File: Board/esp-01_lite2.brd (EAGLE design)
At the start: 17.4 x 56.8 mm, 26 parts, among them IC1 TINY13-20SU, K1 setup, K2 reset, X1 235-102, X2 235-102

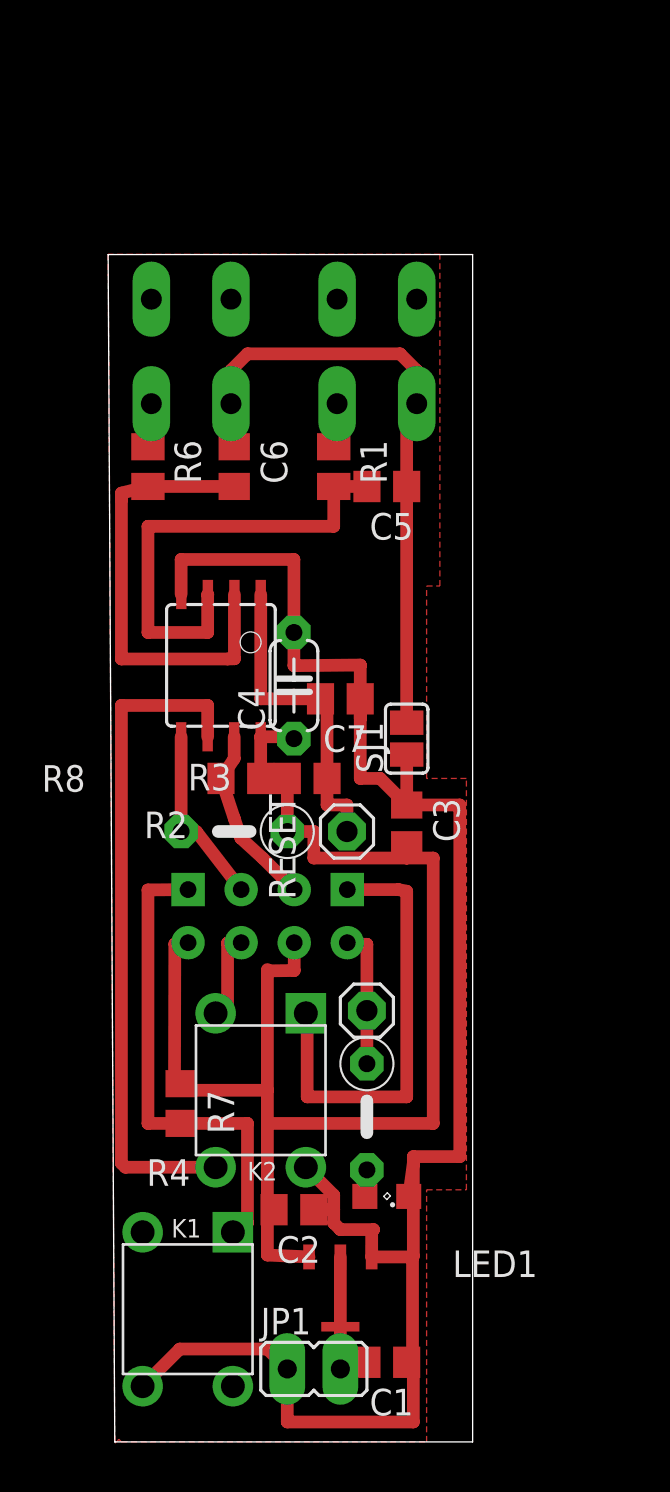
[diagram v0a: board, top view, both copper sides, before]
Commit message: LED works, server ok, ESP 24h
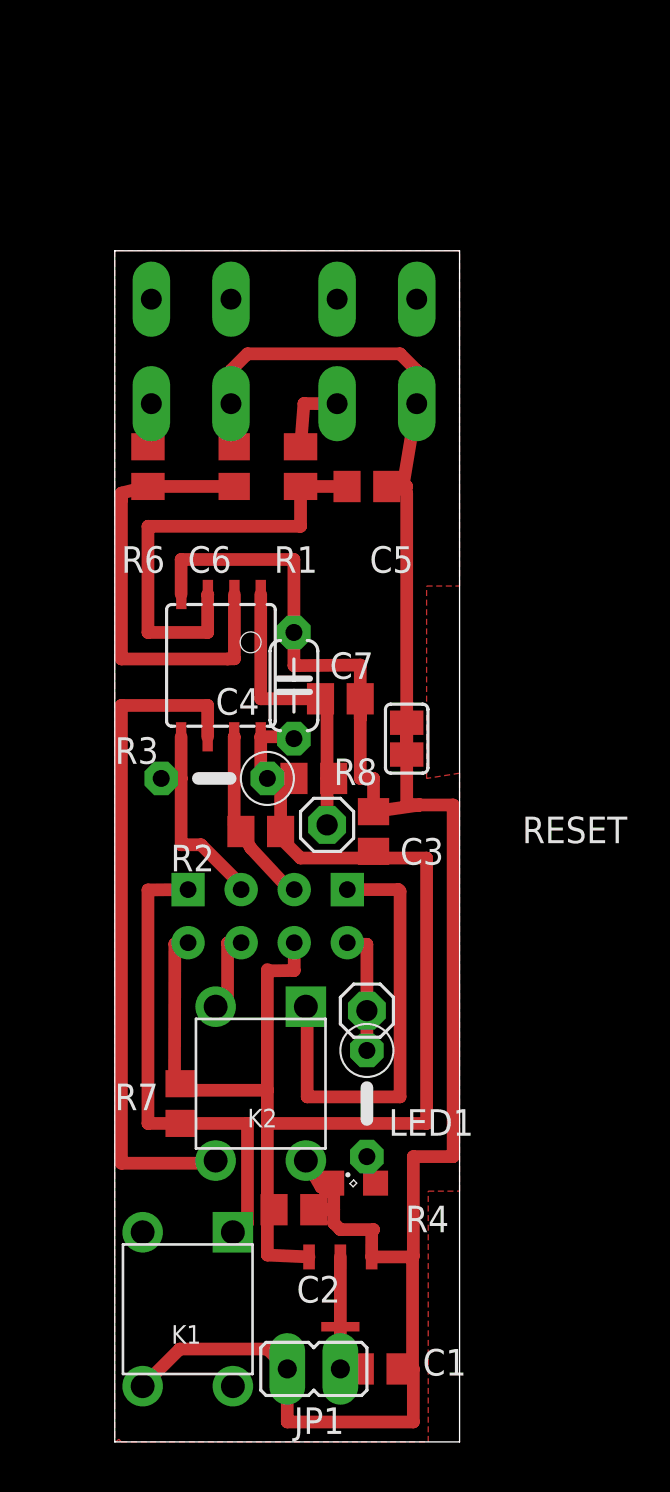
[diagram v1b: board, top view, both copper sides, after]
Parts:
- moved R2 2.71 mm to (6.99, 29.2)
- moved R3 2.71 mm to (4.76, 31.8)
- moved LED1 1.71 mm to (11.4, 12.4), turned to 0 degrees
- moved C3 1.62 mm to (12.4, 29.2)
- moved R1 1.59 mm to (8.89, 46.7)
- moved RESET 1.00 mm to (10.2, 29.5), turned to 90 degrees
- moved C5 0.95 mm to (12.1, 45.7)
- moved R4 0.63 mm to (12.1, 16.2)
- moved C1 0.45 mm to (12.7, 3.49)
- moved R8 0.32 mm to (9.53, 31.8)
- moved K2 0.32 mm to (6.99, 17.1)
- turned SJ1 to 270 degrees
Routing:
- net N$5: track 30.3 -> 34.4 mm
- net GND: track 90.3 -> 93.4 mm
- net N$4: track 2.09 -> 3.66 mm
- net SDA: track 8.77 -> 10.0 mm
- net IN2: track 22.1 -> 21.2 mm
- net N$13: track 16.2 -> 15.2 mm
- net LOG: track 6.66 -> 6.03 mm
- net +3V3: track 68.0 -> 67.4 mm
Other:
- board size 17.4 x 56.8 mm -> 16.5 x 57 mm

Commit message: new board
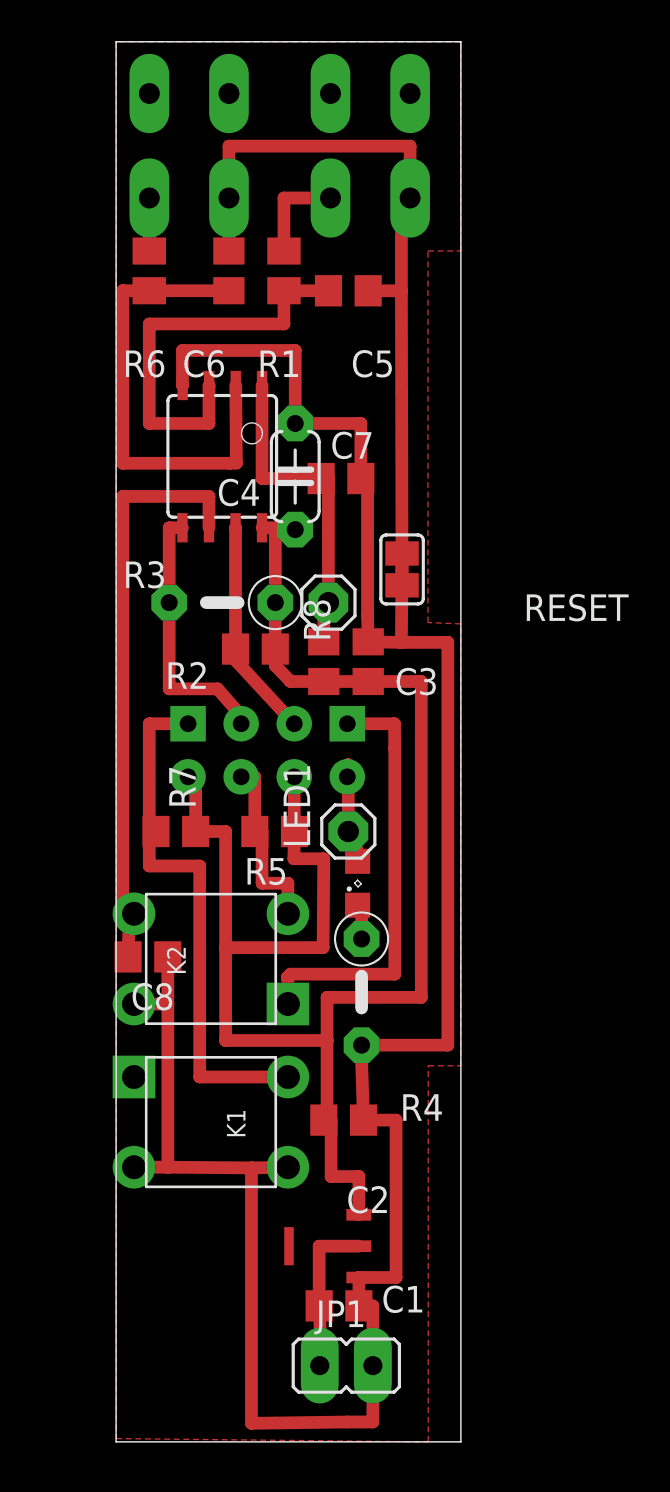
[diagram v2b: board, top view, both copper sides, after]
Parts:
- added C8: 0.1, resistor:C0805
- added R5: 10k, rcl:R0805
- moved LED1 14.4 mm to (11.6, 26.7), turned to 90 degrees
- moved R7 13.0 mm to (2.92, 29.2), turned to 180 degrees
- moved RESET 10.6 mm to (10.2, 40.2)
- moved C7 10.5 mm to (10.8, 46.1)
- moved C4 10.0 mm to (8.64, 46.2)
- moved IC1 10.0 mm to (5.14, 47.1)
- moved X2 9.85 mm to (12.4, 62.9)
- moved X1 9.84 mm to (3.71, 62.9)
- moved C5 9.41 mm to (11.2, 55.1)
- moved R1 9.40 mm to (8.10, 56.0)
- moved C6 9.37 mm to (5.46, 56.0)
- moved R6 9.37 mm to (1.65, 56.0)
- moved K1 9.02 mm to (4.60, 15.3), turned to 0 degrees
- moved R2 8.73 mm to (6.73, 37.9)
- moved LOG 8.62 mm to (11.2, 29.2)
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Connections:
- removed net LOG: LOG.1, R4.1, U$1.TX
- removed net N$12: LED1.A, R4.2
- new net N$1: LED1.A, LOG.1, U$1.TX
- new net N$6: LED1.C, R4.1
- net +3V3: now also R5.1
- net GND: now also C8.1, K1.2, R4.2; no longer LED1.C
- net N$2: now also R5.2
- net RX: now also K1.4; no longer K1.1
- net WAKE_UP: now also C8.2
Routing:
- net GND: track 93.4 -> 114.9 mm
- net +3V3: track 67.4 -> 81.7 mm
- net LOG: track 6.03 -> 0.00 mm
- net N$1: track 0.00 -> 5.31 mm
- net N$2: track 4.34 -> 8.79 mm
- net WAKE_UP: track 32.1 -> 28.4 mm
- net SDA: track 10.0 -> 12.7 mm
- net N$5: track 34.4 -> 36.7 mm
- net RX: track 23.5 -> 25.7 mm
- net SCK: track 8.72 -> 10.5 mm
- net N$6: track 0.00 -> 1.69 mm
- net IN2: track 21.2 -> 19.6 mm
- net AA*3: track 6.31 -> 7.71 mm
- net N$12: track 1.35 -> 0.00 mm
- net N$4: track 3.66 -> 4.76 mm
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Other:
- board size 16.5 x 57 mm -> 16.5 x 67 mm

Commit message: board for one_button
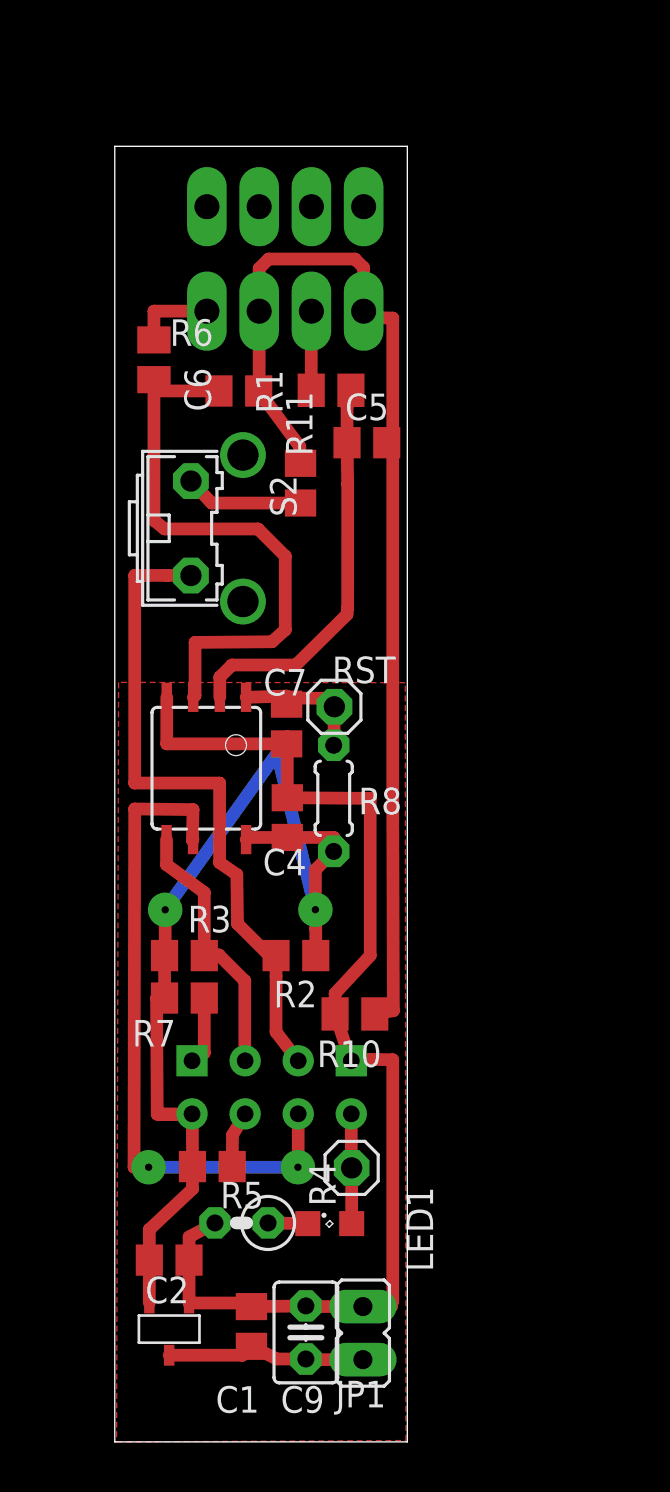
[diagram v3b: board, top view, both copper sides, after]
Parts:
- removed C3, C8: 0.1, resistor:C0805
- removed K1: setup, Seeed-OPL-Button:SW4-6.0X6.0X5.0MM
- removed K2: reset, Seeed-OPL-Button:SW4-6.0X6.0X5.0MM
- removed RESET: RESET, pinhead:1X01
- removed SJ1: (no value), jumper:SJ
- removed X1, X2: 235-102, con-wago_235:P-235-102
- added C9: 10mkF, rcl:C025-030X050
- added R10: 3k3, resistor:M0805
- added R11: 200, rcl:R0805
- added RST: RST, pinhead:1X01
- added S2: (no value), switch-omron:B3F-31XX
- added X3: (no value), con-wago255:233-104
- C4: device resistor:C050-024X044 -> rcl:C0805
- R3: device resistor:0207/5V -> rcl:R0805
- R4: device resistor:0207/5V -> rcl:0207/2V
- R5: value 10k -> 3k3
- R8: value 10k -> 3k3; device rcl:R0805 -> rcl:0204/5
- U$2: value HT7333 -> MCP1700T-3302E/TT; device HT7333_SOT89:SOT89 -> MCP1700T-3302E_TT:MCP1700T-3302E/TT
- moved R3 17.0 mm to (3.33, 23.3), turned to 0 degrees
- moved LED1 16.3 mm to (10.3, 10.4), turned to 0 degrees
- moved C4 16.3 mm to (8.26, 29.9)
- moved R5 16.3 mm to (4.67, 13.2), turned to 0 degrees
- moved U$1 16.1 mm to (7.49, 23.9)
- moved LOG 16.1 mm to (11.3, 13.1)
- moved IC1 14.9 mm to (4.38, 32.2)
- moved R2 14.8 mm to (8.67, 23.3)
- moved R4 12.5 mm to (6.06, 10.5), turned to 180 degrees
- moved C7 12.0 mm to (8.22, 34.4), turned to 90 degrees
- moved C2 10.7 mm to (2.60, 8.70), turned to 0 degrees
- moved U$2 9.36 mm to (2.60, 5.40), turned to 180 degrees
- moved R7 7.98 mm to (3.33, 21.2), turned to 0 degrees
- moved C5 7.32 mm to (12.1, 47.8)
- moved R8 6.56 mm to (10.5, 30.8)
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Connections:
- removed net N$5: C5.1, C6.1, SJ1.2, X1.L1.2, X2.L1.2
- new net N$11: R5.2, U$1.RST
- net +3V3: now also C2.1; no longer C2.2, C3.2, U$1.CH_PD
- net AA*3: now also C1.1, C9.1; no longer C1.2
- net GND: now also C1.2, C2.2, C9.2, R10.2, U$1.GND; no longer C1.1, C2.1, C3.1, C8.1, K1.2, K1.3, K2.4, SJ1.1
- net GND1: now also C5.1, C6.1, R10.1, R11.2, X3.A2, X3.A4; no longer K2.1, U$1.GND
- net IN1: now also C5.2, R1.2; no longer C6.2, R6.2
- net IN2: now also C6.2, R6.2; no longer C5.2, R1.2
- net N$13: now also RST.1; no longer RESET.1
- net N$2: now also R11.1, S2.1; no longer K2.2, R5.2, U$1.RST
- net N$3: now also X3.A1; no longer X1.L2.2
- net N$4: now also X3.A3; no longer X2.L2.2
- net RX: no longer K1.4
- net SCK: now also S2.2
- net WAKE_UP: now also U$1.CH_PD; no longer C8.2, K2.3
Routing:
- net GND: track 114.9 -> 57.6 mm
- net N$5: track 36.7 -> 0.00 mm
- net GND1: track 20.7 -> 53.5 mm
- net +3V3: track 81.7 -> 51.0 mm, vias 0 -> 2
- net RX: track 25.7 -> 3.32 mm
- net SCK: track 10.5 -> 31.7 mm
- net IN2: track 19.6 -> 28.1 mm
- net N$13: track 15.6 -> 7.44 mm
- net WAKE_UP: track 28.4 -> 31.9 mm, vias 0 -> 2
- net IN1: track 22.5 -> 19.0 mm
- net N$2: track 8.79 -> 5.70 mm
- net N$11: track 0.00 -> 2.69 mm
- net AA*3: track 7.71 -> 9.99 mm
- net N$3: track 2.54 -> 3.92 mm
- net N$4: track 4.76 -> 3.79 mm
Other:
- board size 16.5 x 67 mm -> 14 x 62 mm
